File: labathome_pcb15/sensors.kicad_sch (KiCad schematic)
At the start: 31 parts, among them J16 BME280, J17 CCS811, J21 QWIIC, U12 BME680, U13 BME280, U15 CCS811, U19 DS18B20, U20 BH1750, U22 AM612, U23 MPU-6050, U26 MSM261D4030H1CPM, U3 AHT21, U7 DS18B20, X2 XGZP6897D

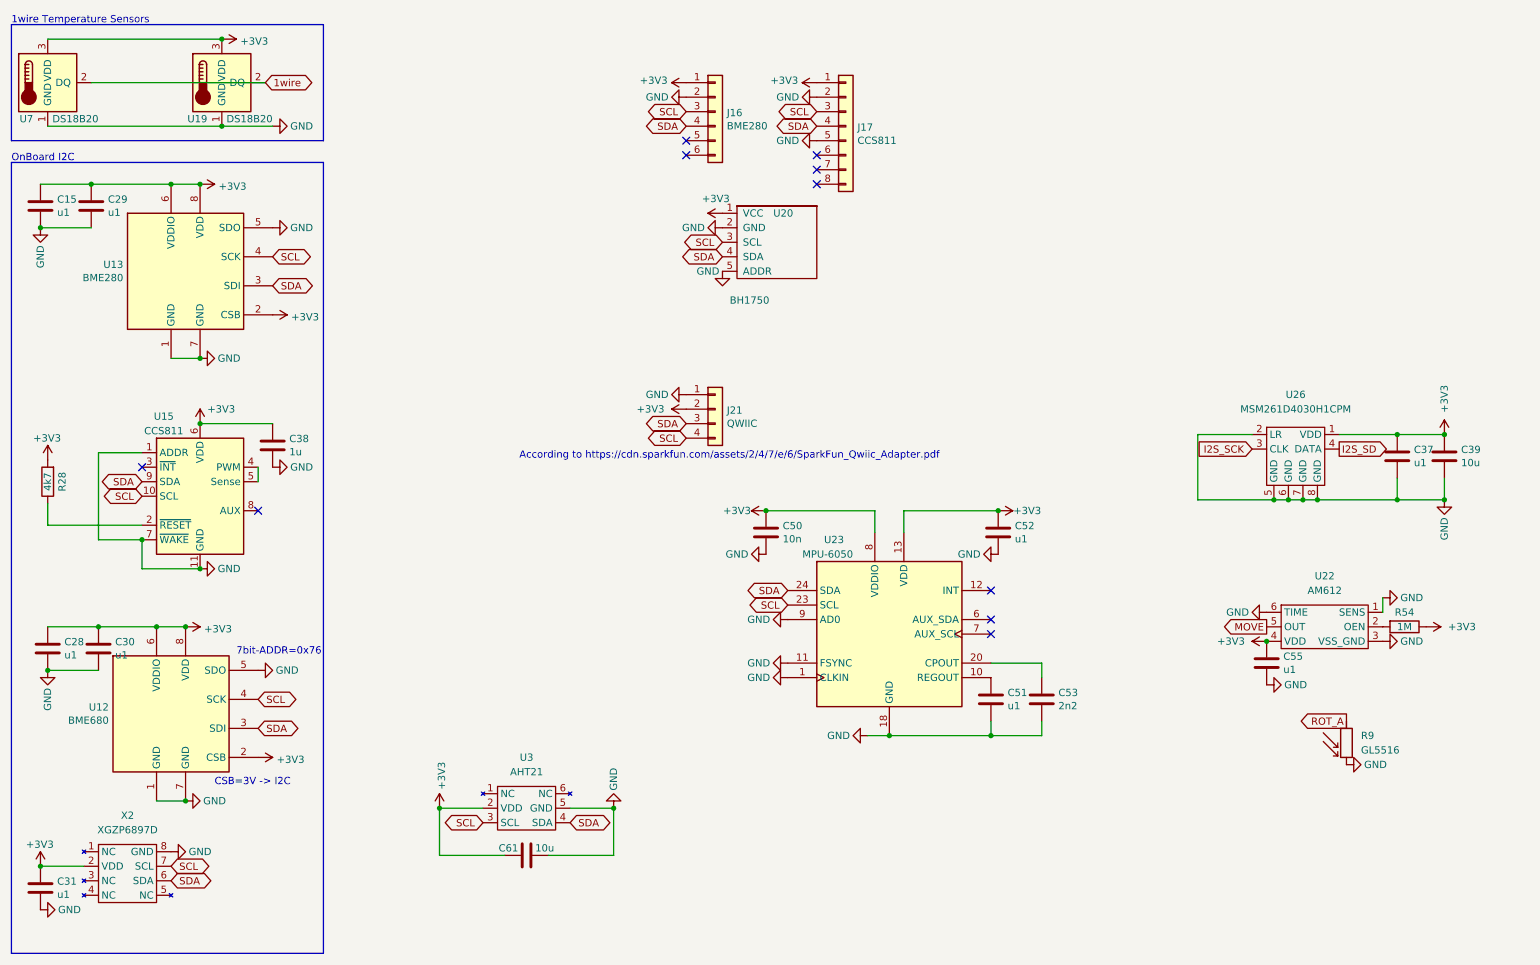
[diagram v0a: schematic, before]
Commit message: PCB_v15 wip
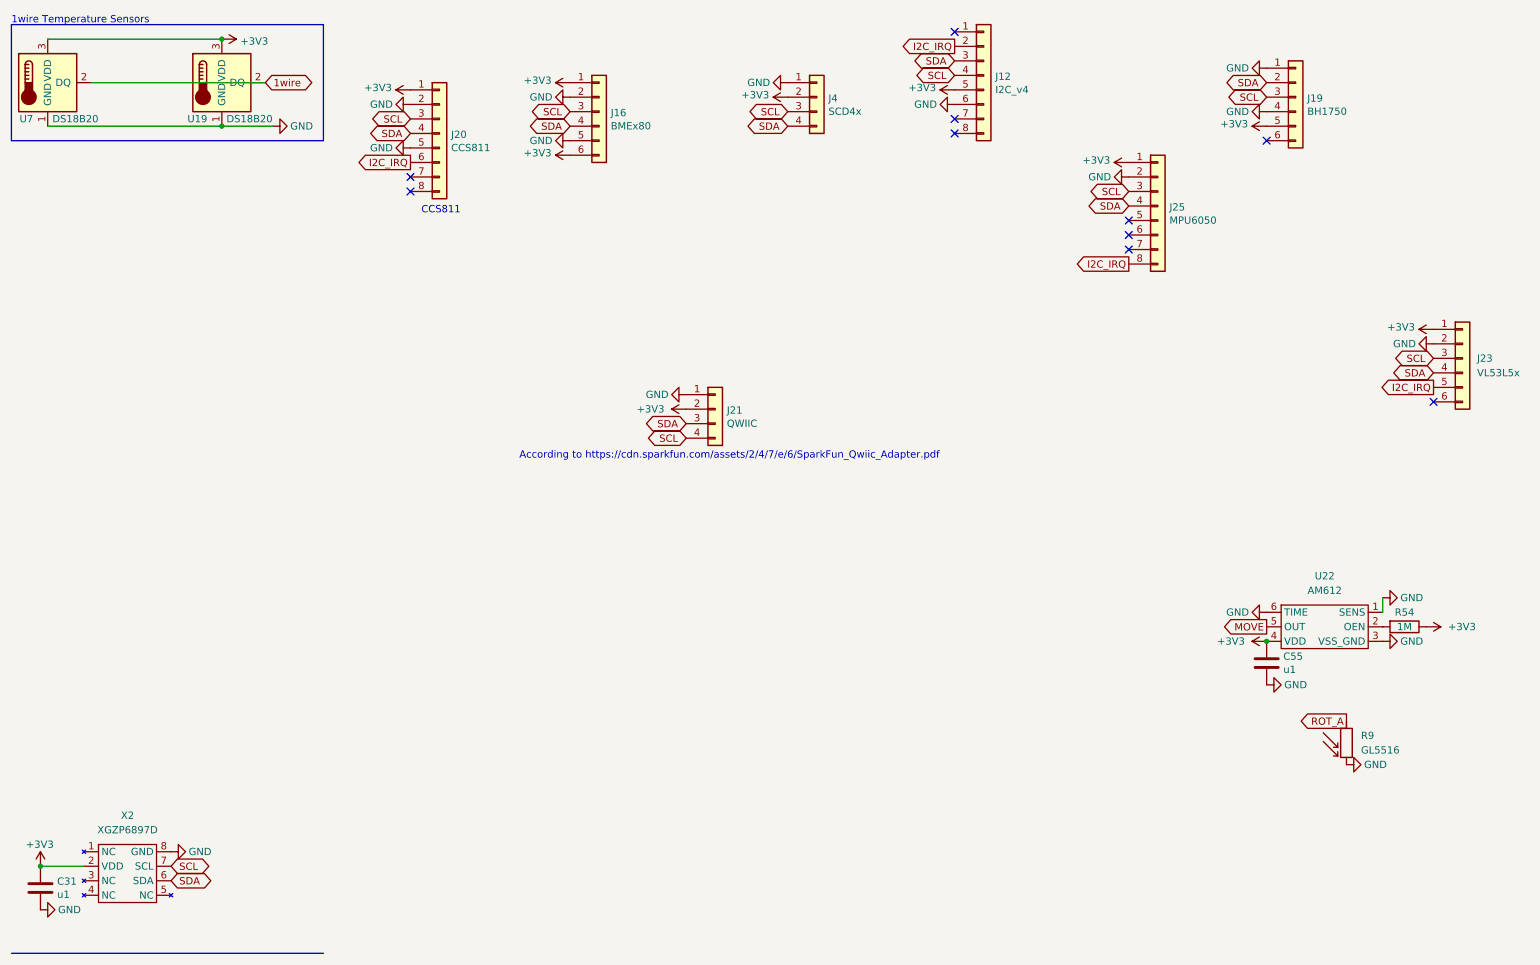
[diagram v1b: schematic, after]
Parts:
- removed C15, C28, C29, C30, C37, C51, C52: u1, Capacitor_SMD:C_0603_1608Metric, symbol Device:C
- removed C38: 1u, Capacitor_SMD:C_0603_1608Metric, symbol Device:C
- removed C39, C61: 10u, Capacitor_SMD:C_0603_1608Metric, symbol Device:C
- removed C50: 10n, Capacitor_SMD:C_0603_1608Metric, symbol Device:C
- removed C53: 2n2, Capacitor_SMD:C_0603_1608Metric, symbol Device:C
- removed J17: CCS811, Connector_PinSocket_2.54mm:PinSocket_1x08_P2.54mm_Vertical, symbol Connector_Generic:Conn_01x08
- removed R28: 4k7, Resistor_SMD:R_0603_1608Metric, symbol Device:R
- removed U12: BME680, Package_LGA:Bosch_LGA-8_3x3mm_P0.8mm_ClockwisePinNumbering, symbol Sensor:BME680
- removed U13: BME280, Package_LGA:Bosch_LGA-8_2.5x2.5mm_P0.65mm_ClockwisePinNumbering, symbol Sensor:BME280
- removed U15: CCS811, liebler_SEMICONDUCTORS:AMS_LGA-10-1EP_2.7x4mm_P0.6mm, symbol Sensor_Gas:CCS811
- removed U20: BH1750, liebler_MODULES:GY-302, symbol smopla:GY-302
- removed U23: MPU-6050, Sensor_Motion:InvenSense_QFN-24_4x4mm_P0.5mm, symbol Sensor_Motion:MPU-6050
- removed U26: MSM261D4030H1CPM, liebler_SEMICONDUCTORS:MSM261D4030H1CPM, symbol liebler_SEMICONDUCTORS:MSM261D4030H1CPM
- removed U3: AHT21, liebler_SEMICONDUCTORS:AHT21, symbol liebler_SEMICONDUCTORS:AHT21
- added J12: I2C_v4, Connector_PinSocket_2.54mm:PinSocket_1x08_P2.54mm_Vertical, symbol Connector_Generic:Conn_01x08
- added J19: BH1750, Connector_PinSocket_2.54mm:PinSocket_1x06_P2.54mm_Vertical, symbol Connector_Generic:Conn_01x06
- added J20: CCS811, Connector_PinSocket_2.54mm:PinSocket_1x08_P2.54mm_Vertical, symbol Connector_Generic:Conn_01x08
- added J23: VL53L5x, Connector_PinSocket_2.54mm:PinSocket_1x06_P2.54mm_Vertical, symbol Connector_Generic:Conn_01x06
- added J25: MPU6050, Connector_PinSocket_2.54mm:PinSocket_1x08_P2.54mm_Vertical, symbol Connector_Generic:Conn_01x08
- added J4: SCD4x, Connector_PinSocket_2.54mm:PinSocket_1x04_P2.54mm_Vertical, symbol Connector_Generic:Conn_01x04
- J16: value BME280 -> BMEx80
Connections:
- net +3V3: now also J16.6 (Pin_6), J12.5 (Pin_5), J19.5 (Pin_5), J20.1 (Pin_1), J23.1 (Pin_1), J25.1 (Pin_1), J4.2 (Pin_2)
- net GND: now also J16.5 (Pin_5), J12.6 (Pin_6), J19.1 (Pin_1), J19.4 (Pin_4), J20.2 (Pin_2), J20.5 (Pin_5), J23.2 (Pin_2), J25.2 (Pin_2), J4.1 (Pin_1)
- net SCL: now also J12.4 (Pin_4), J19.3 (Pin_3), J20.3 (Pin_3), J23.3 (Pin_3), J25.3 (Pin_3), J4.3 (Pin_3)
- net SDA: now also J12.3 (Pin_3), J19.2 (Pin_2), J20.4 (Pin_4), J23.4 (Pin_4), J25.4 (Pin_4), J4.4 (Pin_4)
- new net I2C_IRQ: J12.2 (Pin_2), J20.6 (Pin_6), J23.5 (Pin_5), J25.8 (Pin_8)
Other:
- note added: "CCS811"
- note removed: "7bit-ADDR=0x76"
- note removed: "CSB=3V -> I2C"
- note removed: "OnBoard I2C"
- moved on the sheet: J16

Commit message: pcb15 WIP
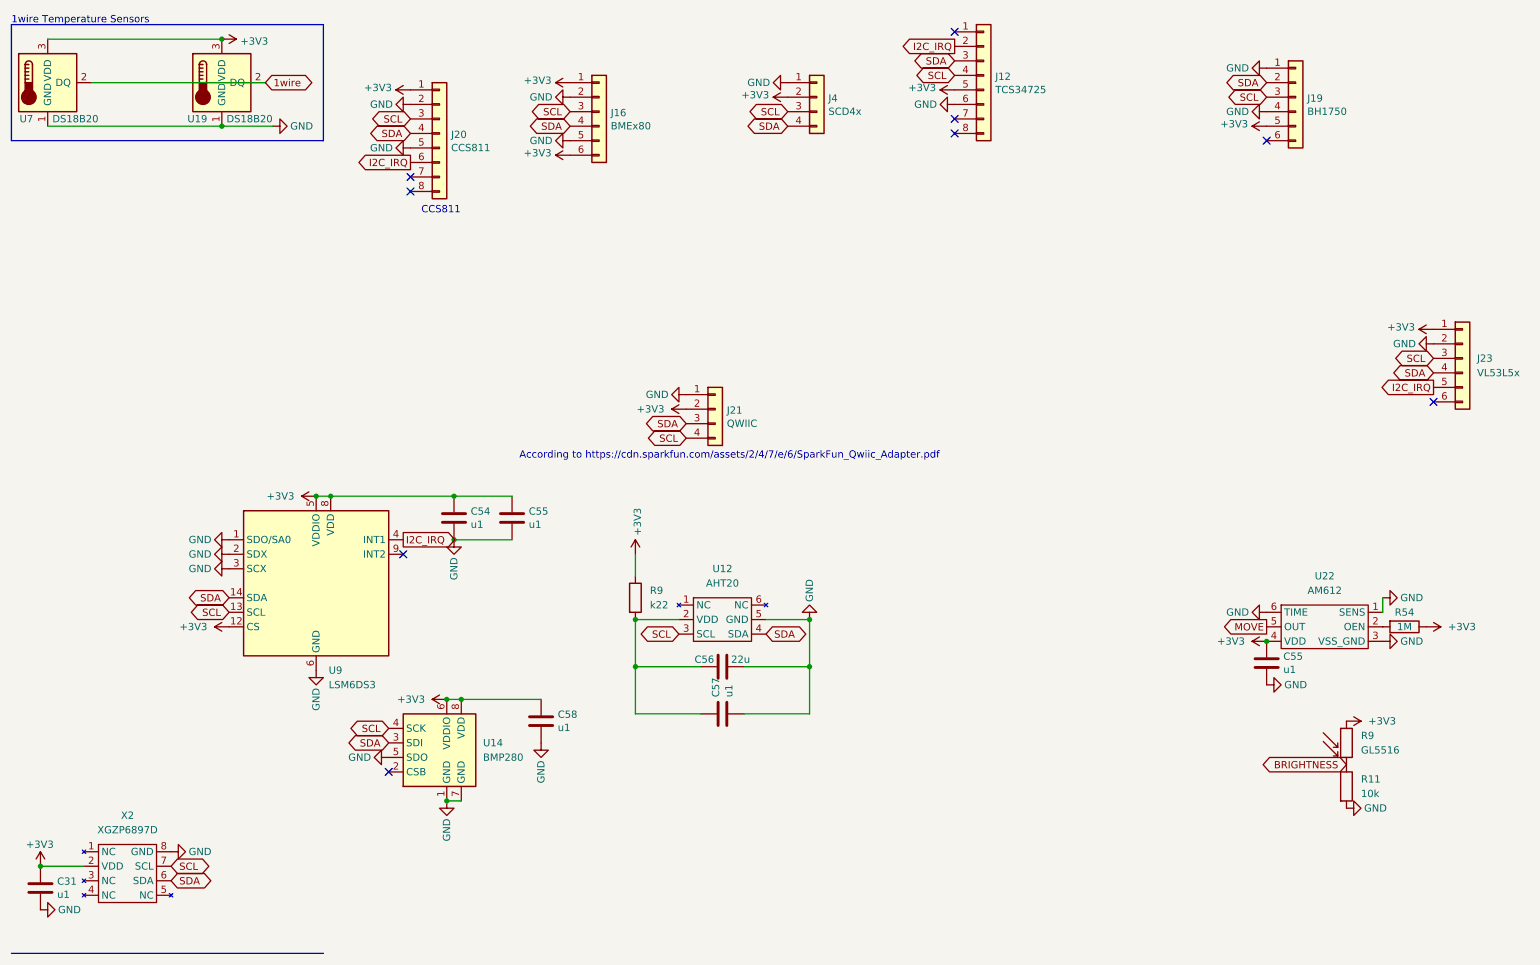
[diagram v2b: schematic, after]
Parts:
- removed J25: MPU6050, Connector_PinSocket_2.54mm:PinSocket_1x08_P2.54mm_Vertical, symbol Connector_Generic:Conn_01x08
- added C54, C55, C57, C58: u1, Capacitor_SMD:C_0402_1005Metric, symbol Device:C
- added C56: 22u, Capacitor_SMD:C_0603_1608Metric, symbol Device:C
- added R11: 10k, Resistor_SMD:R_0402_1005Metric, symbol Device:R
- added R9: k22, Resistor_SMD:R_0402_1005Metric, symbol Device:R
- added U12: AHT20, liebler_SEMICONDUCTORS:AHT21, symbol liebler_SEMICONDUCTORS:AHT21
- added U14: BMP280, Package_LGA:Bosch_LGA-8_2x2.5mm_P0.65mm_ClockwisePinNumbering, symbol Sensor_Pressure:BMP280
- added U9: LSM6DS3, Package_LGA:LGA-14_3x2.5mm_P0.5mm_LayoutBorder3x4y, symbol Sensor_Motion:LSM6DS3
- J12: value I2C_v4 -> TCS34725
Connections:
- net ROT_A is gone; now on net +3V3: R9.1
- net +3V3: now also C54.2, C55.2, C58.2, R9.1, U14.6 (VDDIO), U14.8 (VDD), U9.12 (CS), U9.5 (VDDIO), U9.8 (VDD)
- net GND: now also C54.1, C55.1, C56.2, C57.1, C58.1, R11.2, U12.5 (GND), U14.1 (GND), U14.5 (SDO), U14.7 (GND), U9.1 (SDO/SA0), U9.2 (SDX), U9.3 (SCX), U9.6 (GND), U9.7 (GND); no longer R9.2
- net I2C_IRQ: now also U9.4 (INT1)
- net SCL: now also U12.3 (SCL), U14.4 (SCK), U9.13 (SCL)
- net SDA: now also U12.4 (SDA), U14.3 (SDI), U9.14 (SDA)
- new net: C56.1, C57.2, R9.2, U12.2 (VDD)
- new net BRIGHTNESS: R11.1, R9.2
- no-connect marks 10 -> 9

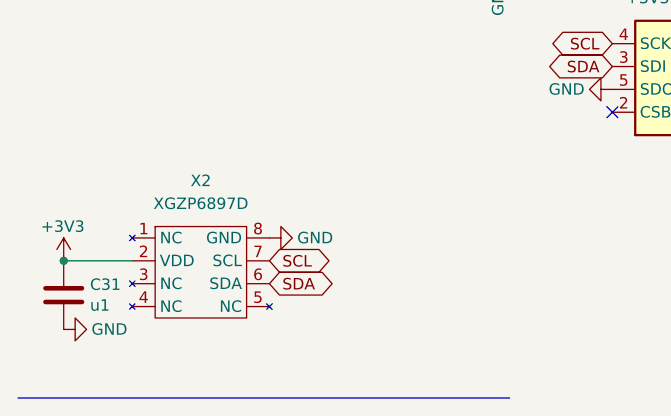
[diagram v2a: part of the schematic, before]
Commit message: labathome wip
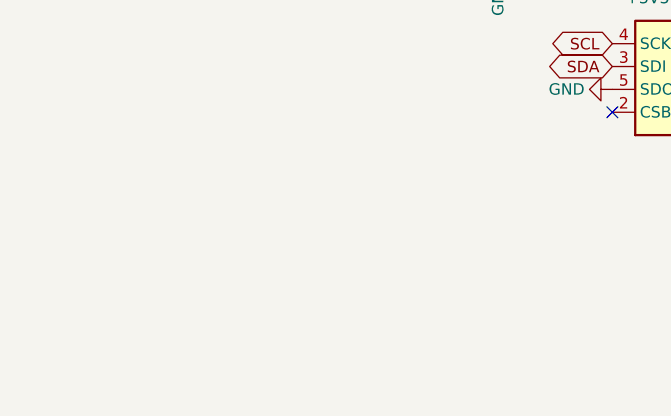
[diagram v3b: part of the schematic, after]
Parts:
- removed C31: u1, Capacitor_SMD:C_0603_1608Metric, symbol Device:C
- removed X2: XGZP6897D, liebler_MODULES:XGZP6897D, symbol liebler_MODULES:XGZP6897D
